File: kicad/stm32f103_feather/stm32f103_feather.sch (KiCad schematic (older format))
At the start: 36 parts, among them J1 Bottom-conn, J2 Top-conn, J3 Debug-conn, J4 USB_B_Micro, J5 JST-LiPo-conn, Q1 SI2301CDS, SW1 SW_Push, U1 STM32F103CBTx, U2 AMS1117-3.3, U3 MCP73831-2-OT, Y1 8MHz

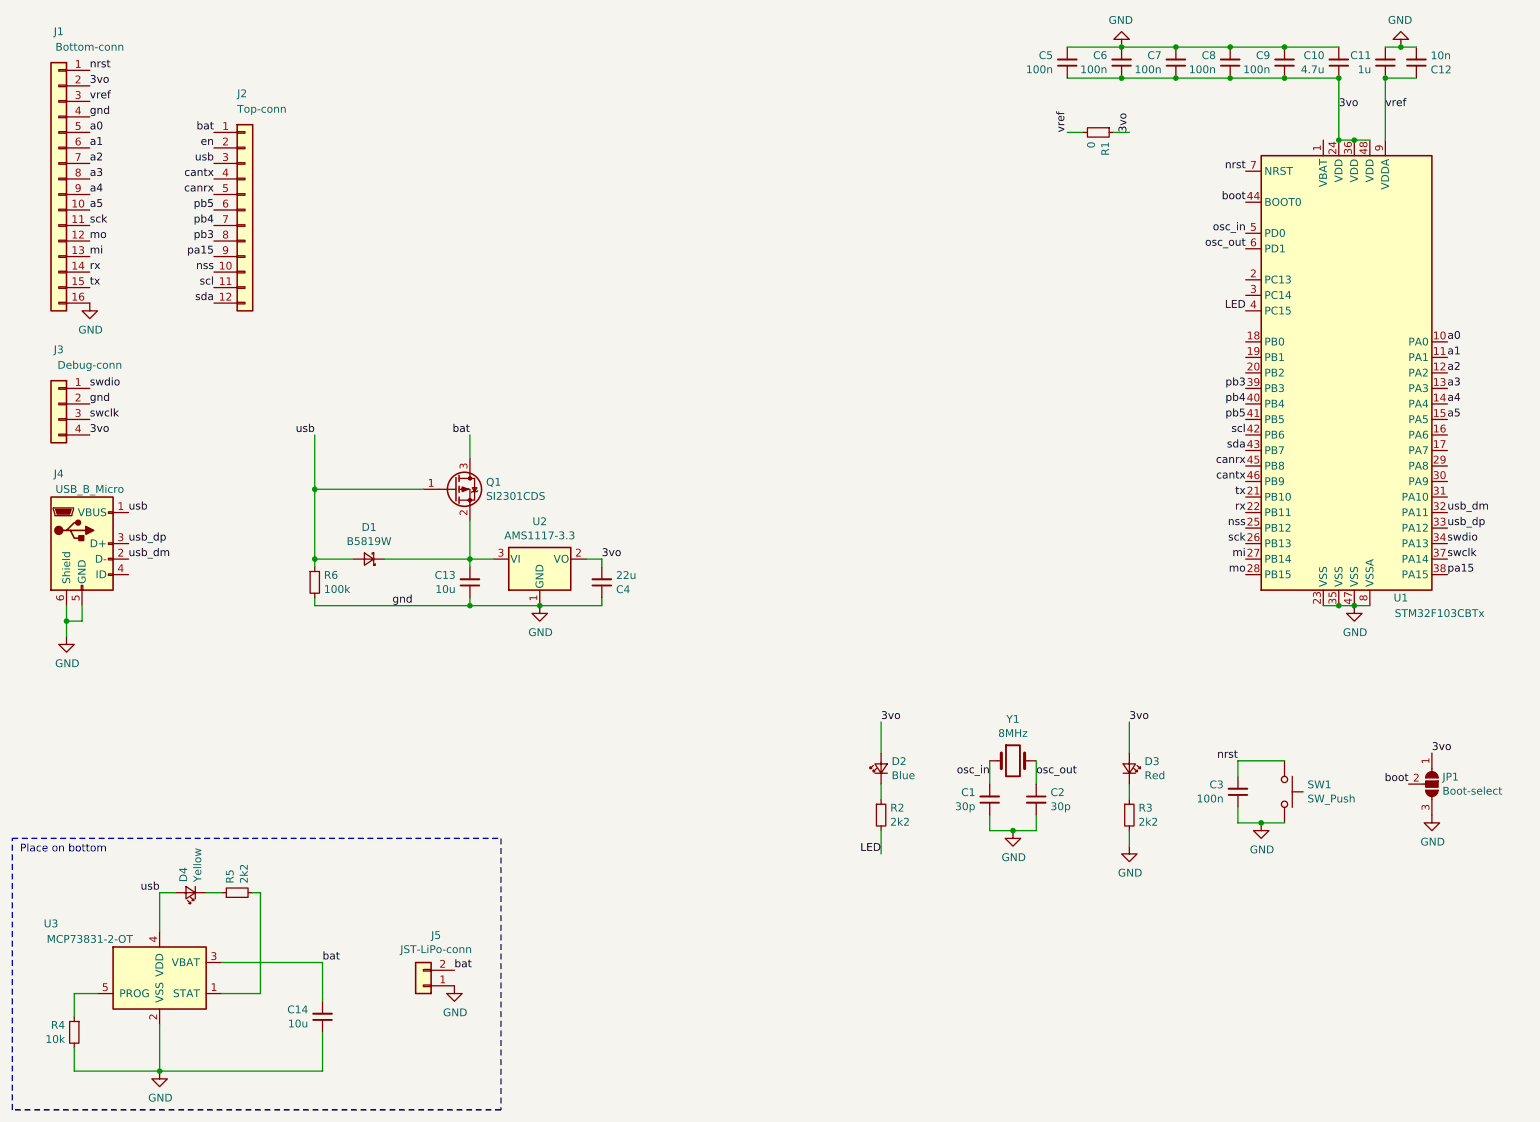
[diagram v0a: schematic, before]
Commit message: daily updates
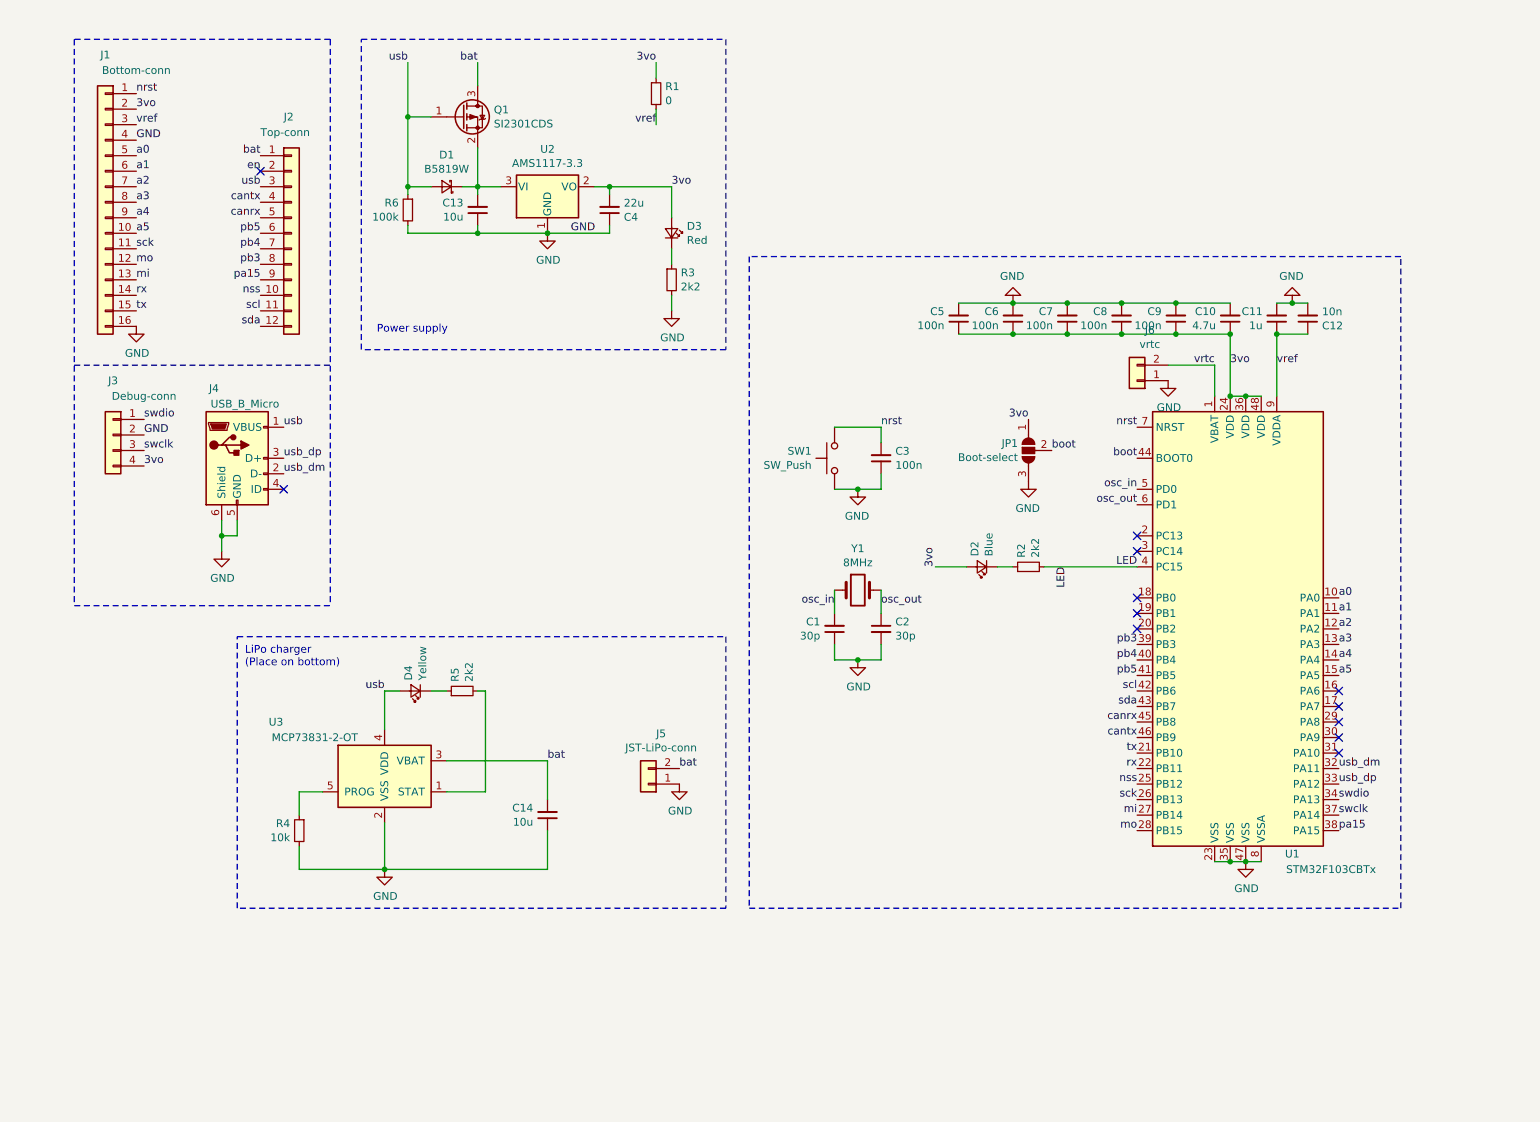
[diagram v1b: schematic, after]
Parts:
- added J6: vrtc, Resistor_SMD:R_0402_1005Metric, symbol Connector_Generic:Conn_01x02
- C11, C12, C14: footprint Capacitor_SMD:C_0603_1608Metric_Pad1.05x0.95mm_HandSolder -> Capacitor_SMD:C_0805_2012Metric_Pad1.15x1.40mm_HandSolder
- D4: footprint Diode_SMD:D_0603_1608Metric_Pad1.05x0.95mm_HandSolder -> Diode_SMD:D_0805_2012Metric_Pad1.15x1.40mm_HandSolder
- R4, R5: footprint Resistor_SMD:R_0603_1608Metric_Pad1.05x0.95mm_HandSolder -> Resistor_SMD:R_0805_2012Metric_Pad1.15x1.40mm_HandSolder
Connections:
- net GND: now also J6.1 (Pin_1)
- net vrtc: now reaches U1.1 (VBAT)
- net vrtc: now also J6.2 (Pin_2)
- no-connect marks 0 -> 12
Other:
- note added: "LiPo charger\n(Place on bottom)"
- note added: "Power supply"
- note removed: "Place on bottom"
- moved on the sheet: C1, C10, C11, C12, C13, C14, C2, C3, C4, C5, C6, C7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

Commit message: daily updates
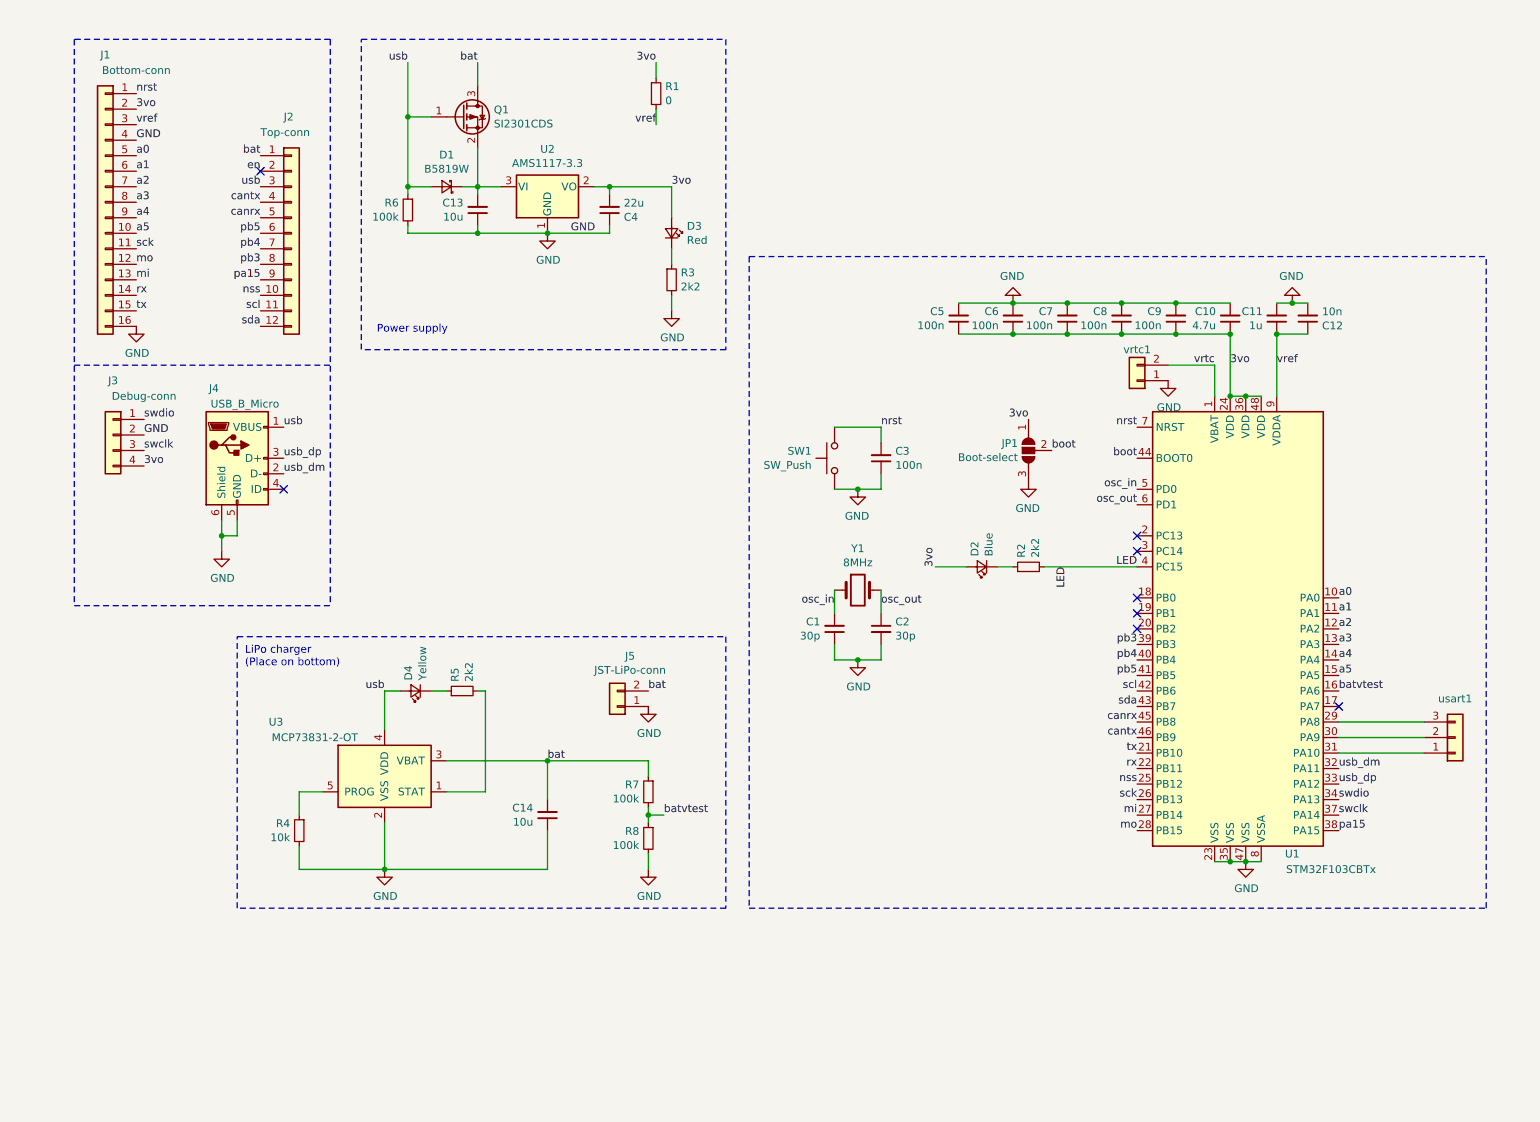
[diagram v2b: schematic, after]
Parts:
- added R7, R8: 100k, Resistor_SMD:R_0805_2012Metric_Pad1.15x1.40mm_HandSolder, symbol Device:R_Small
- added usart1: Conn_01x03, Jumper:SolderJumper-3_P1.3mm_Open_Pad1.0x1.5mm, symbol Connector_Generic:Conn_01x03
- renumbered J6 to vrtc1
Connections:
- net GND: now also R8.2
- net bat: now also R7.1
- net batvtest: now reaches U1.16 (PA6)
- net batvtest: now also R7.2, R8.1
- net at U1.29 (PA8): now also usart1.3 (Pin_3)
- net at U1.30 (PA9): now also usart1.2 (Pin_2)
- net at U1.31 (PA10): now also usart1.1 (Pin_1)
- no-connect marks 12 -> 8
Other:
- moved on the sheet: J5
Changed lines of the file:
@@
 Text Label 2550 3550 0    50   ~ 0
-usb_dm
-Text Label 9350 5450 0    50   ~ 0
 usb_dm
 $Comp
@@
 L power:GND #PWR0110
 U 1 1 5F3F0470
-P 5100 5550
-F 0 "#PWR0110" H 5100 5300 50  0001 C CNN
-F 1 "GND" H 5105 5377 50  0000 C CNN
-F 2 "" H 5100 5550 50  0001 C CNN
-F 3 "" H 5100 5550 50  0001 C CNN
-	1    5100 5550
-	1    0    0    -1
-$EndComp
-Text Label 5100 5450 0    50   ~ 0
+P 4900 5050
+F 0 "#PWR0110" H 4900 4800 50  0001 C CNN
+F 1 "GND" H 4905 4877 50  0000 C CNN
+F 2 "" H 4900 5050 50  0001 C CNN
+F 3 "" H 4900 5050 50  0001 C CNN
+	1    4900 5050
+	1    0    0    -1
+$EndComp
+Text Label 4900 4950 0    50   ~ 0
 bat
 $Comp
 L Connector_Generic:Conn_01x02 J5
 U 1 1 5F3A21F3
-P 4900 5550
-F 0 "J5" H 4818 5225 50  0000 C CNN
-F 1 "JST-LiPo-conn" H 4818 5316 50  0000 C CNN
-F 2 "Connector_JST:JST_PH_S2B-PH-SM4-TB_1x02-1MP_P2.00mm_Horizontal" H 4900 5550 50  0001 C CNN
-F 3 "~" H 4900 5550 50  0001 C CNN
-	1    4900 5550
+P 4700 5050
+F 0 "J5" H 4618 4725 50  0000 C CNN
+F 1 "JST-LiPo-conn" H 4618 4816 50  0000 C CNN
+F 2 "Connector_JST:JST_PH_S2B-PH-SM4-TB_1x02-1MP_P2.00mm_Horizontal" H 4700 5050 50  0001 C CNN
+F 3 "~" H 4700 5050 50  0001 C CNN
+	1    4700 5050
 	-1   0    0    1
 $EndComp
@@
 Wire Wire Line
 	8850 3050 8750 3050
-$Comp
-L MCU_ST_STM32F1:STM32F103CBTx U1
-U 1 1 5F3A98EE
-P 8750 4550
-F 0 "U1" H 9050 3100 50  0000 C CNN
-F 1 "STM32F103CBTx" H 9300 3000 50  0000 C CNN
-F 2 "Package_QFP:LQFP-48_7x7mm_P0.5mm" H 8150 3150 50  0001 R CNN
-F 3 "http://www.st.com/st-web-ui/static/active/en/resource/technical/document/datasheet/CD00161566.pdf" H 8750 4550 50  0001 C CNN
-F 4 "C8304" H 8750 4550 50  0001 C CNN "LSCS"
-	1    8750 4550
-	1    0    0    -1
-$EndComp
 Text Label 9350 5850 0    50   ~ 0
 pa15
@@
 Power supply
 Wire Notes Line
-	9750 6350 9750 2150
-Wire Notes Line
-	9750 2150 5550 2150
+	10300 6350 10300 2150
 Wire Notes Line
 	5550 2150 5550 6350
 Wire Notes Line
-	5550 6350 9750 6350
-Wire Notes Line
 	1200 2850 2850 2850
 Wire Notes Line
@@
 Wire Wire Line
 	3700 1700 3800 1700
-NoConn ~ 9350 5350
-NoConn ~ 9350 5250
-NoConn ~ 9350 5150
 NoConn ~ 9350 5050
-NoConn ~ 9350 4950
 NoConn ~ 8050 4550
 NoConn ~ 8050 4450
@@
 vrtc
 $Comp
-L Connector_Generic:Conn_01x02 J6
+L Connector_Generic:Conn_01x02 vrtc1
 U 1 1 5F4EC4D8
 P 8050 2950
-F 0 "J6" H 7968 2625 50  0000 C CNN
-F 1 "vrtc" H 7968 2716 50  0000 C CNN
+F 0 "vrtc1" H 8050 2750 50  0000 C CNN
+F 1 "vrtc" H 7968 2716 50  0001 C CNN
 F 2 "Resistor_SMD:R_0402_1005Metric" H 8050 2950 50  0001 C CNN
 F 3 "~" H 8050 2950 50  0001 C CNN
@@
 NoConn ~ 2550 3650
 NoConn ~ 2400 1600
+$Comp
+L Device:R_Small R7
+U 1 1 5F3D06A1
+P 4900 5600
+F 0 "R7" H 4959 5646 50  0000 L CNN
+F 1 "100k" H 4959 5555 50  0000 L CNN
+F 2 "Resistor_SMD:R_0805_2012Metric_Pad1.15x1.40mm_HandSolder" H 4900 5600 50  0001 C CNN
+F 3 "~" H 4900 5600 50  0001 C CNN
+F 4 "C25804" H 4900 5600 50  0001 C CNN "LCSC"
+	1    4900 5600
+	-1   0    0    -1
+$EndComp
+$Comp
+L Device:R_Small R8
+U 1 1 5F3D0C34
+P 4900 5900
+F 0 "R8" H 4959 5946 50  0000 L CNN
+F 1 "100k" H 4959 5855 50  0000 L CNN
+F 2 "Resistor_SMD:R_0805_2012Metric_Pad1.15x1.40mm_HandSolder" H 4900 5900 50  0001 C CNN
+F 3 "~" H 4900 5900 50  0001 C CNN
+F 4 "C25804" H 4900 5900 50  0001 C CNN "LCSC"
+	1    4900 5900
+	-1   0    0    -1
+$EndComp
+$Comp
+L power:GND #PWR0114
+U 1 1 5F3D132A
+P 4900 6100
+F 0 "#PWR0114" H 4900 5850 50  0001 C CNN
+F 1 "GND" H 4905 5927 50  0000 C CNN
+F 2 "" H 4900 6100 50  0001 C CNN
+F 3 "" H 4900 6100 50  0001 C CNN
+	1    4900 6100
+	1    0    0    -1
+$EndComp
+Wire Wire Line
+	4900 5500 4900 5400
+Wire Wire Line
+	4900 5400 4250 5400
+Connection ~ 4250 5400
+Wire Wire Line
+	4900 6000 4900 6100
+Text Label 5000 5750 0    50   ~ 0
+batvtest
+Wire Wire Line
+	4900 5700 4900 5750
+Wire Wire Line
+	5000 5750 4900 5750
+Connection ~ 4900 5750
+Wire Wire Line
+	4900 5750 4900 5800
+Text Label 9350 4950 0    50   ~ 0
+batvtest
+$Comp
+L Connector_Generic:Conn_01x03 usart1
+U 1 1 5F3DF3AE
+P 10100 5250
+F 0 "usart1" H 10100 5000 50  0000 C CNN
+F 1 "Conn_01x03" H 10018 5016 50  0001 C CNN
+F 2 "Jumper:SolderJumper-3_P1.3mm_Open_Pad1.0x1.5mm" H 10100 5250 50  0001 C CNN
+F 3 "~" H 10100 5250 50  0001 C CNN
+	1    10100 5250
+	1    0    0    1
+$EndComp
+Text Label 9350 5450 0    50   ~ 0
+usb_dm
+$Comp
+L MCU_ST_STM32F1:STM32F103CBTx U1
+U 1 1 5F3A98EE
+P 8750 4550
+F 0 "U1" H 9050 3100 50  0000 C CNN
+F 1 "STM32F103CBTx" H 9300 3000 50  0000 C CNN
+F 2 "Package_QFP:LQFP-48_7x7mm_P0.5mm" H 8150 3150 50  0001 R CNN
+F 3 "http://www.st.com/st-web-ui/static/active/en/resource/technical/document/datasheet/CD00161566.pdf" H 8750 4550 50  0001 C CNN
+F 4 "C8304" H 8750 4550 50  0001 C CNN "LSCS"
+	1    8750 4550
+	1    0    0    -1
+$EndComp
+Wire Wire Line
+	9350 5150 9900 5150
+Wire Wire Line
+	9900 5250 9350 5250
+Wire Wire Line
+	9350 5350 9900 5350
+Wire Notes Line
+	5550 6350 10300 6350
+Wire Notes Line
+	5550 2150 10300 2150
 $EndSCHEMATC
